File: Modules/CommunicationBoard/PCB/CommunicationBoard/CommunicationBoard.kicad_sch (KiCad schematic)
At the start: 12 parts, among them J1 CIO_MAIN_CONNECTOR, J2 Conn_Coaxial, U1 E22-900M30S

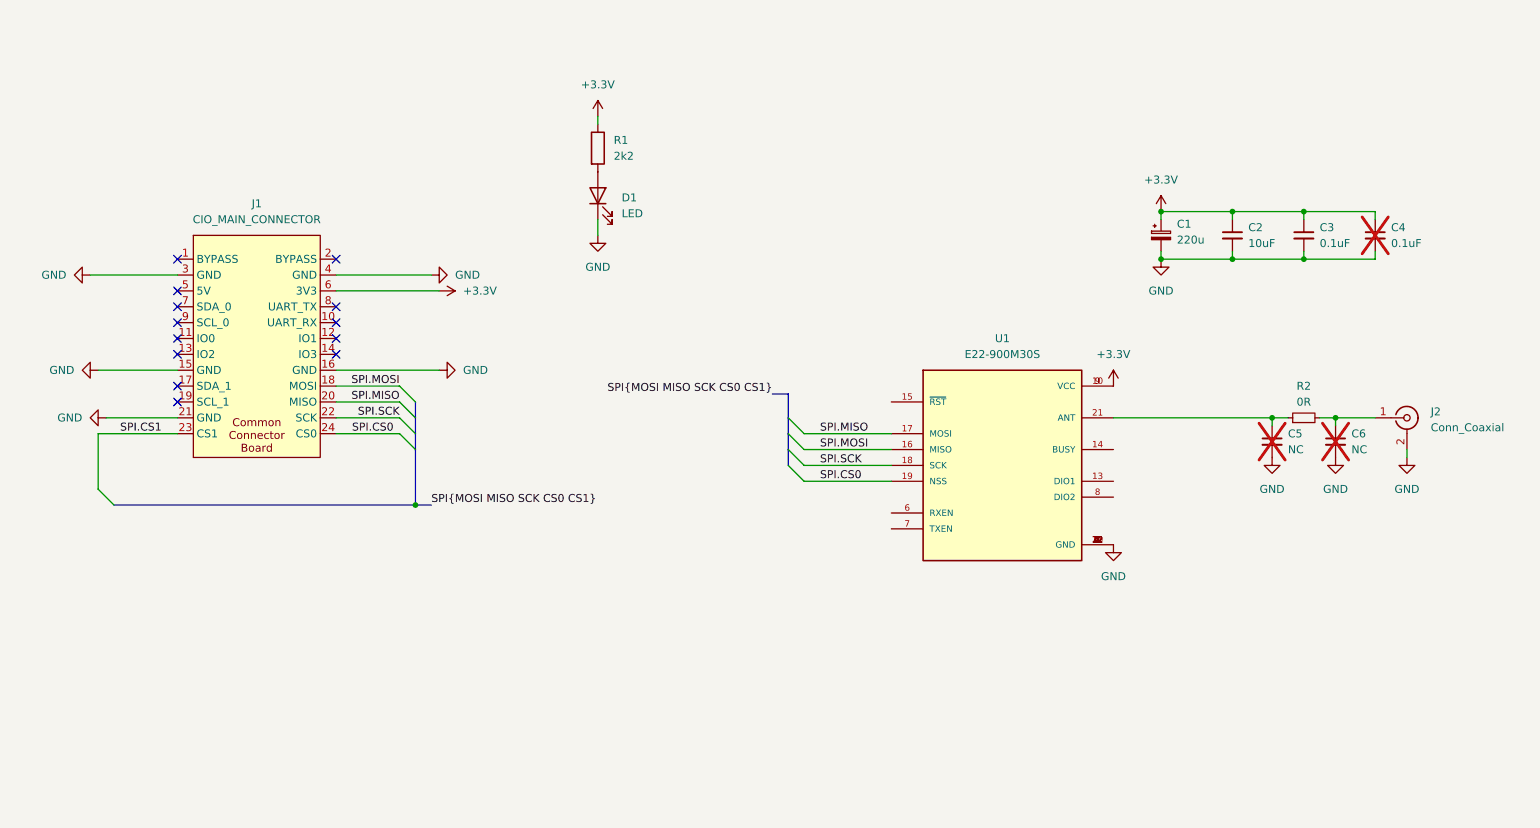
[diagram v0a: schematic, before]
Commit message: First PCB layout version
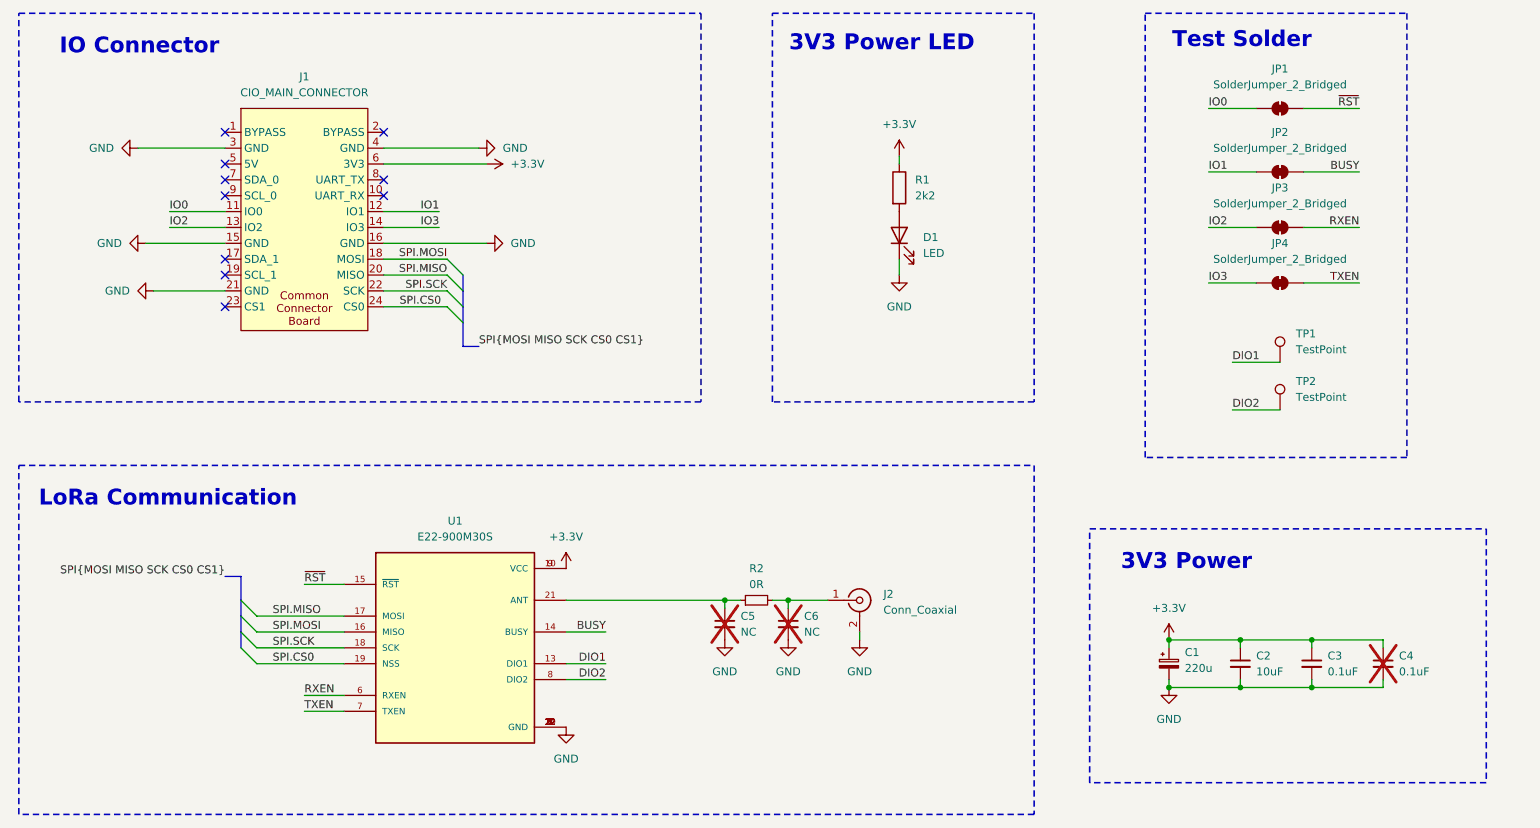
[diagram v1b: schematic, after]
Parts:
- added JP1, JP2, JP3, JP4: SolderJumper_2_Bridged, Jumper:SolderJumper-2_P1.3mm_Bridged_RoundedPad1.0x1.5mm, symbol Jumper:SolderJumper_2_Bridged
- added TP1, TP2: TestPoint, TestPoint:TestPoint_Pad_D2.5mm, symbol Connector:TestPoint
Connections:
- net DIO1: now reaches U1.13 (DIO1)
- net DIO1: now also TP1.1
- net BUSY: now reaches U1.14 (BUSY)
- net BUSY: now also JP2.2 (B)
- net ~{RST}: now reaches U1.15 (~{RST})
- net ~{RST}: now also JP1.2 (B)
- net RXEN: now reaches U1.6 (RXEN)
- net RXEN: now also JP3.2 (B)
- net TXEN: now reaches U1.7 (TXEN)
- net TXEN: now also JP4.2 (B)
- net DIO2: now reaches U1.8 (DIO2)
- net DIO2: now also TP2.1
- net IO0: now reaches J1.11 (IO0)
- net IO0: now also JP1.1 (A)
- net IO1: now reaches J1.12 (IO1)
- net IO1: now also JP2.1 (A)
- net IO2: now reaches J1.13 (IO2)
- net IO2: now also JP3.1 (A)
- net IO3: now reaches J1.14 (IO3)
- net IO3: now also JP4.1 (A)
- net SPI.CS1: no longer names the net of J1.23 (CS1)
- no-connect marks 13 -> 10
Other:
- note added: "3V3 Power"
- note added: "3V3 Power LED"
- note added: "IO Connector"
- note added: "LoRa Communication"
- note added: "Test Solder"
- moved on the sheet: C1, C2, C3, C4, C5, C6, D1, J1, J2, R1, R2, U1
